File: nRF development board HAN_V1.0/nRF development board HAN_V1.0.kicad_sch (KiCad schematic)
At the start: 0 parts

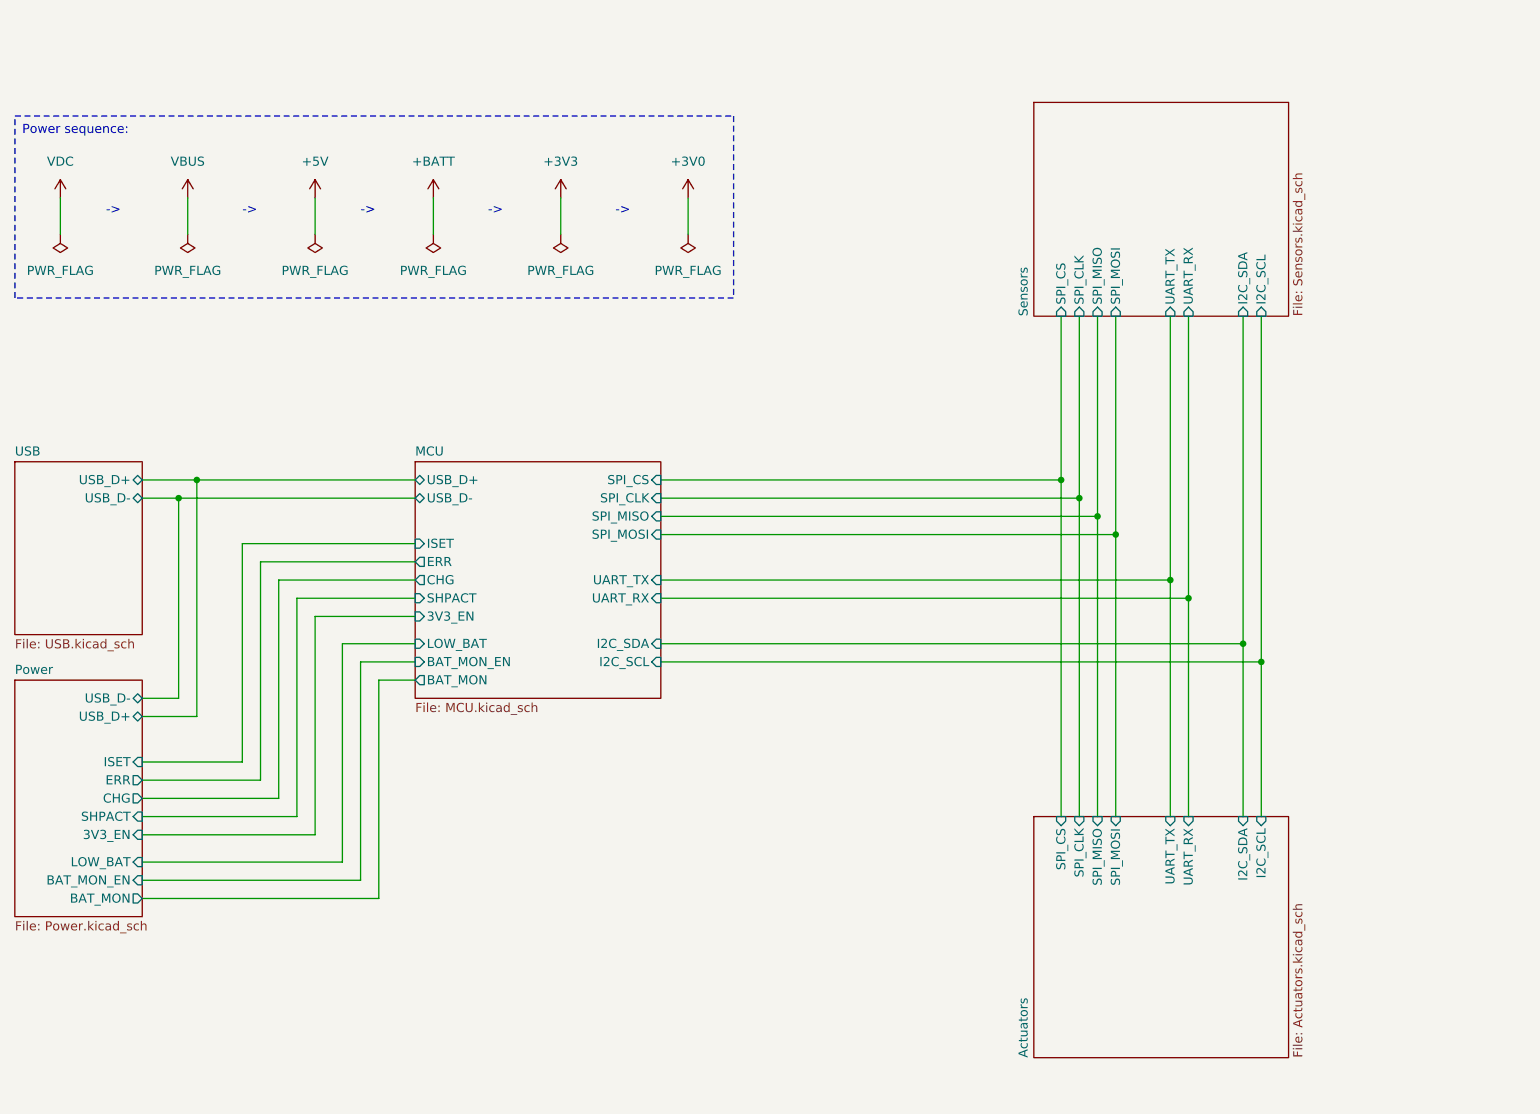
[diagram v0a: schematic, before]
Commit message: Updated schematic
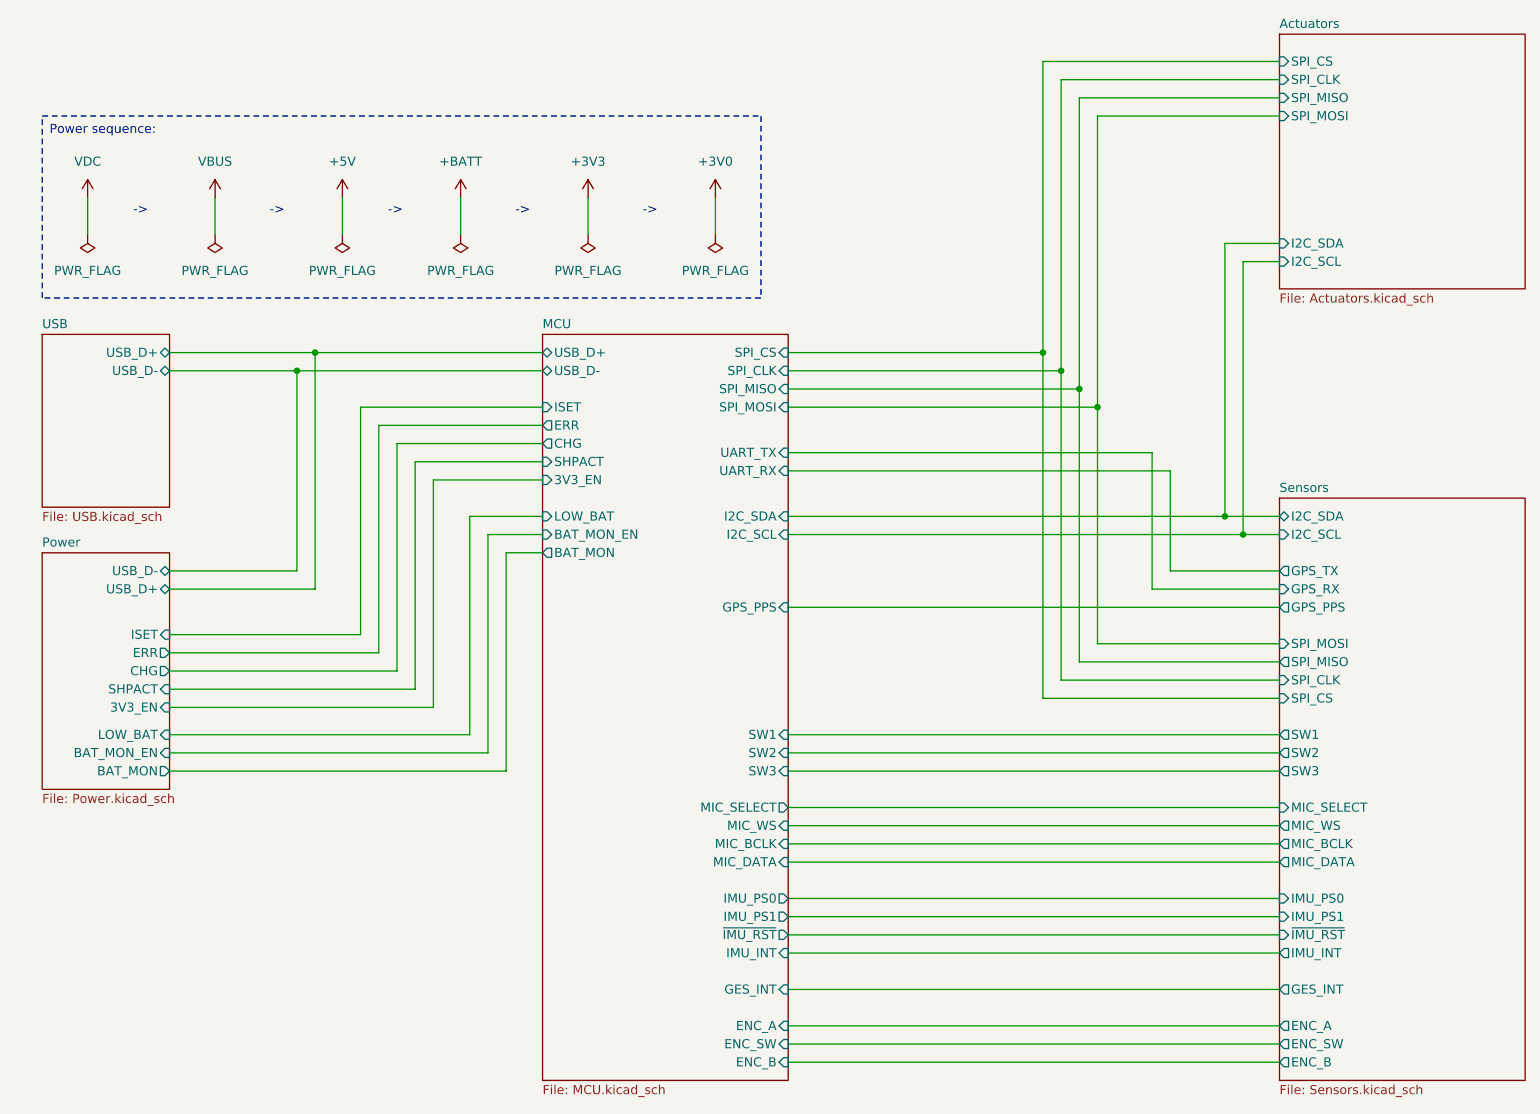
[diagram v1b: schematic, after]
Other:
- sheet Actuators ports: added none; removed UART_RX, UART_TX
- sheet MCU ports: added ENC_A, ENC_B, ENC_SW, GES_INT, GPS_PPS, IMU_INT, IMU_PS0, IMU_PS1, MIC_BCLK, MIC_DATA, MIC_SELECT, MIC_WS, SW1, SW2, SW3, ~{IMU_RST}; removed none
- sheet Sensors ports: added ENC_A, ENC_B, ENC_SW, GES_INT, GPS_PPS, GPS_RX, GPS_TX, IMU_INT, IMU_PS0, IMU_PS1, MIC_BCLK, MIC_DATA, MIC_SELECT, MIC_WS, SW1, SW2, SW3, ~{IMU_RST}; removed UART_RX, UART_TX
